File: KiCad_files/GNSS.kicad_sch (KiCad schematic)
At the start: 12 parts

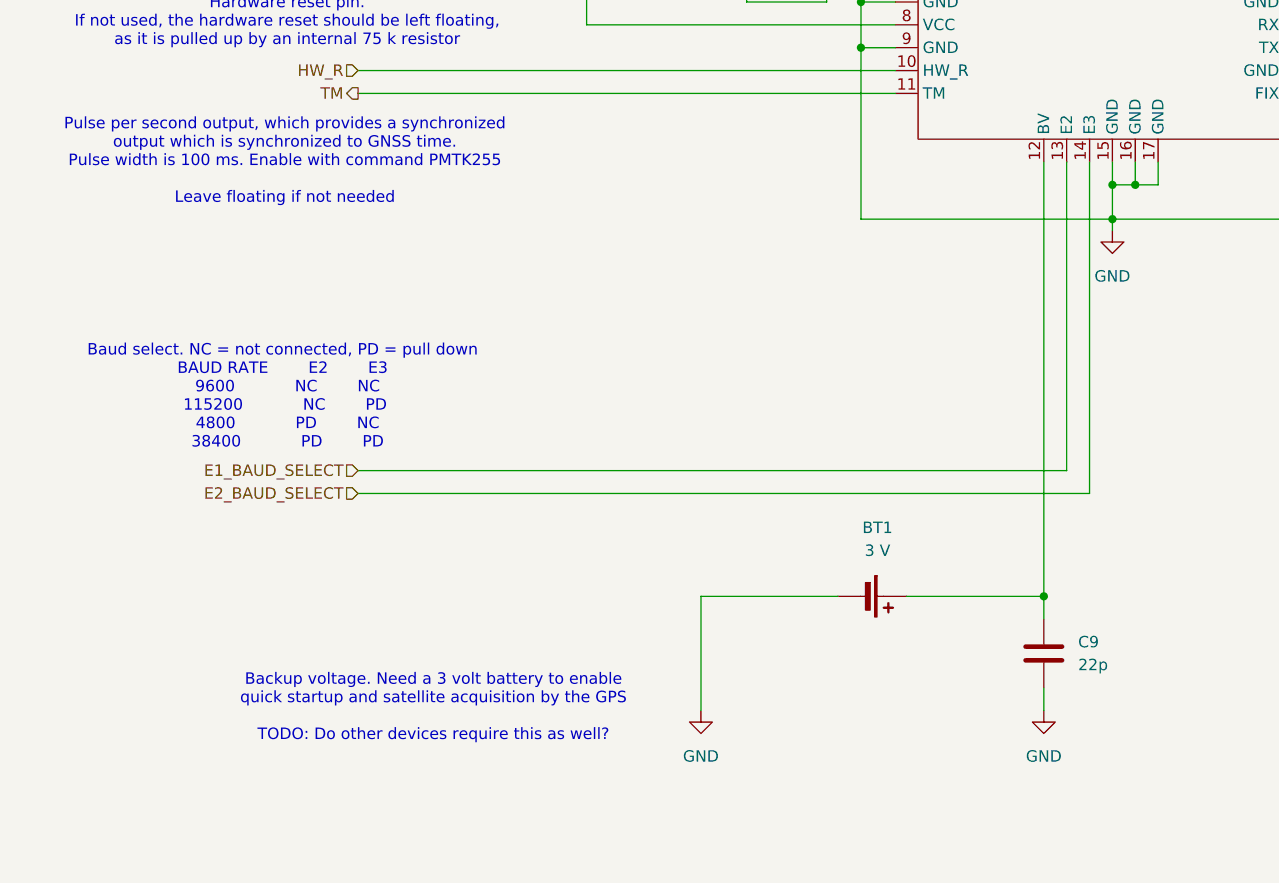
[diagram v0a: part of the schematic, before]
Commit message: paristo lisätty
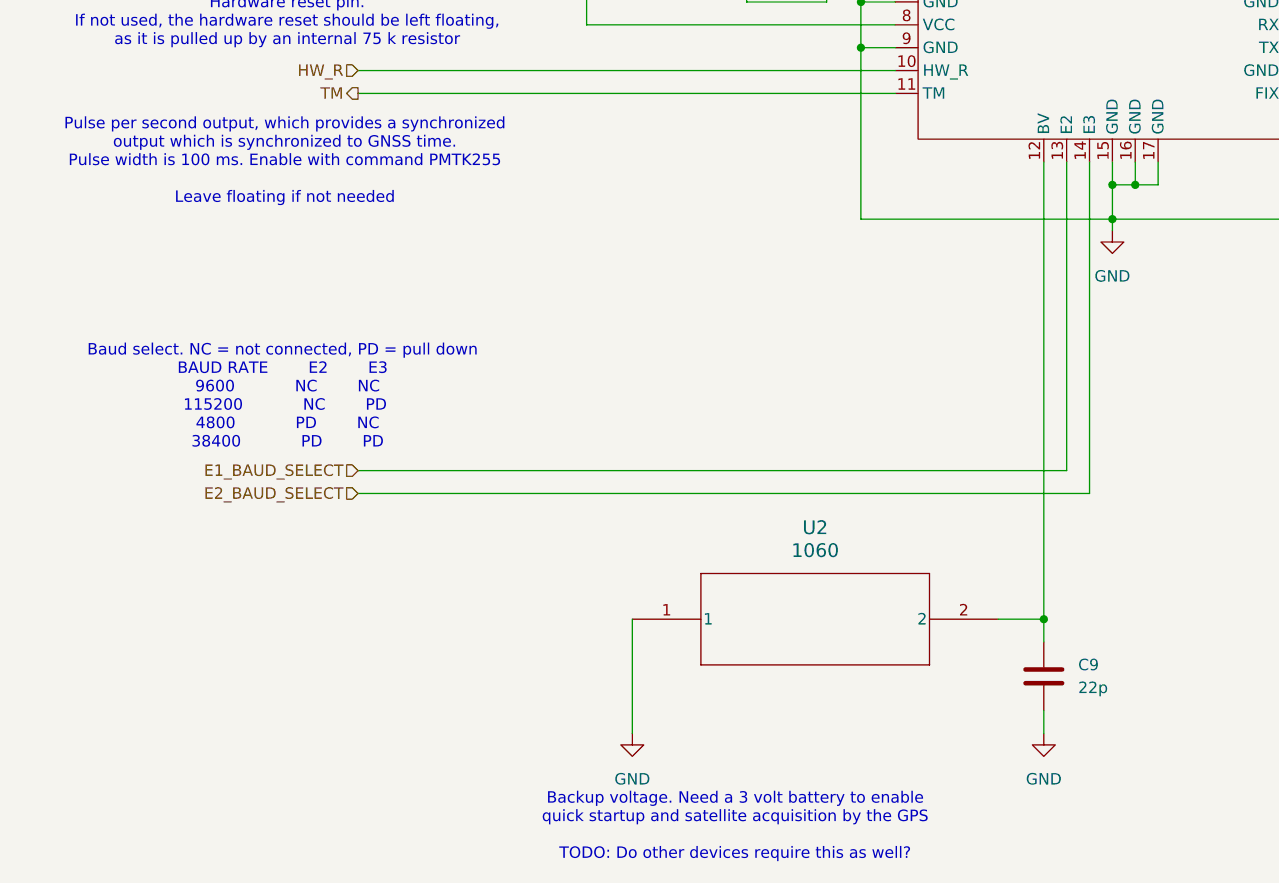
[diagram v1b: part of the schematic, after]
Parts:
- removed BT1: 3 V, symbol Device:Battery_Cell
- added U2: 1060, 1060_KEY, symbol 1_projektin osat:1060
- C10: DigiKey (none) -> 399-C0805C225K4RACTUCT-ND
- C11, C12, C13, C14, C9: DigiKey (none) -> 399-17625-1-ND
- R9: DigiKey (none) -> 311-0.0ARCT-ND
- U10: DigiKey (none) -> 627-1099-1-ND
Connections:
- net GND: now also U2.1
- net at C9.1, U10.12 (BV): now also U2.2
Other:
- moved on the sheet: C9

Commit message: update
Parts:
- U2: footprint 1060_KEY -> 1_project_library:1060_KEY
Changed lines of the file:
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@@
+			)
+		)
+		(property "Sim.Type" ""
+			(at 50.8 69.85 0)
+			(effects
+				(font
+					(size 1.27 1.27)
+				)
+				(hide yes)
 			)
 		)
@@
 			)
 		)
+		(property "Sim.Type" ""
+			(at 93.98 93.98 0)
+			(effects
+				(font
+					(size 1.27 1.27)
+				)
+				(hide yes)
+			)
+		)
 		(pin "2"
 		)
@@
 			)
 		)
+		(property "Sim.Type" ""
+			(at 196.85 104.14 90)
+			(effects
+				(font
+					(size 1.27 1.27)
+				)
+				(hide yes)
+			)
+		)
 		(pin "1"
 		)
@@
 			)
 		)
+		(property "Sim.Type" ""
+			(at 203.2 120.65 0)
+			(effects
+				(font
+					(size 1.27 1.27)
+				)
+				(hide yes)
+			)
+		)
 		(pin "2"
 		)
@@
 			)
 		)
+		(property "Sim.Type" ""
+			(at 63.5 69.85 0)
+			(effects
+				(font
+					(size 1.27 1.27)
+				)
+				(hide yes)
+			)
+		)
 		(pin "2"
 		)
@@
 			)
 		)
+		(property "Sim.Type" ""
+			(at 127 173.99 0)
+			(effects
+				(font
+					(size 1.27 1.27)
+				)
+				(hide yes)
+			)
+		)
 		(pin "1"
 		)
@@
 			)
 		)
+		(property "Sim.Type" ""
+			(at 95.25 62.23 90)
+			(effects
+				(font
+					(size 1.27 1.27)
+				)
+				(hide yes)
+			)
+		)
 		(pin "2"
 		)
@@
 			)
 		)
-		(property "Footprint" "1060_KEY"
+		(property "Footprint" "1_project_library:1060_KEY"
 			(at 81.28 167.64 0)
 			(effects
@@
 			)
 		)
+		(property "Sim.Type" ""
+			(at 81.28 167.64 0)
+			(effects
+				(font
+					(size 1.27 1.27)
+				)
+				(hide yes)
+			)
+		)
 		(pin "1"
 		)
@@
 			)
 		)
+		(property "Sim.Type" ""
+			(at 170.18 62.23 90)
+			(effects
+				(font
+					(size 1.27 1.27)
+				)
+				(hide yes)
+			)
+		)
 		(pin "1"
 		)
@@
 			)
 		)
+		(property "Sim.Type" ""
+			(at 113.03 78.74 0)
+			(effects
+				(font
+					(size 1.27 1.27)
+				)
+				(hide yes)
+			)
+		)
 		(pin "14"
 		)
@@
 			)
 		)
+		(property "Sim.Type" ""
+			(at 184.15 101.6 90)
+			(effects
+				(font
+					(size 1.27 1.27)
+				)
+				(hide yes)
+			)
+		)
 		(pin "1"
 		)
@@
 			(at 190.5 120.65 0)
 			(effects
+				(font
+					(size 1.27 1.27)
+				)
+				(hide yes)
+			)
+		)
+		(property "Sim.Type" ""
+			(at 190.5 120.65 0)
+			(effects
